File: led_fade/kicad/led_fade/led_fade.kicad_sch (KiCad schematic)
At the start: 3 parts

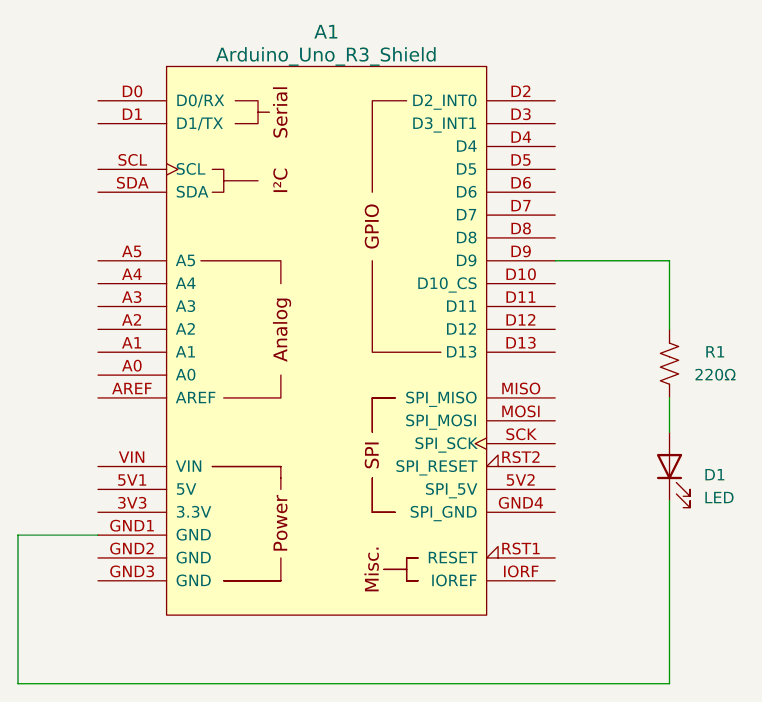
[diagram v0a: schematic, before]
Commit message: Use default Arduino UNO R3 symbol
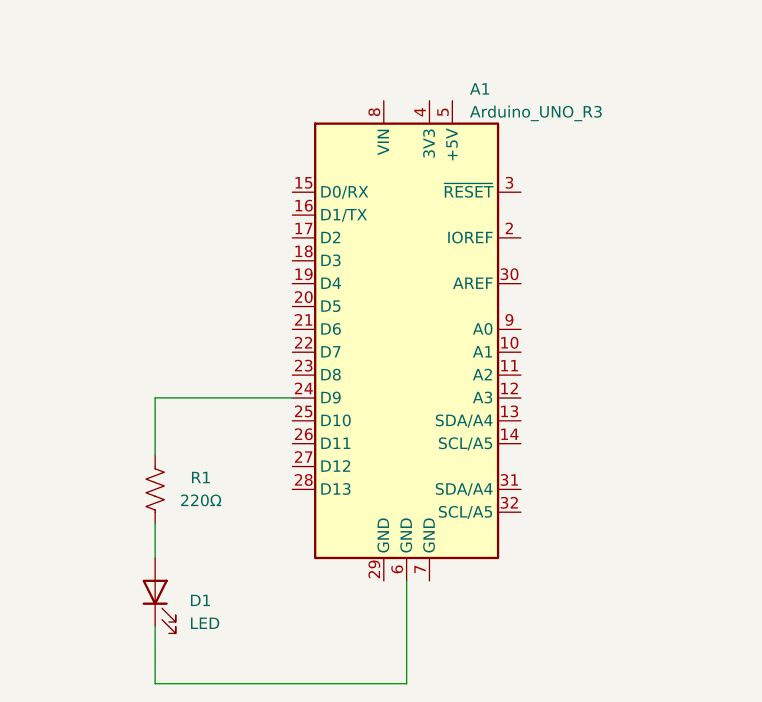
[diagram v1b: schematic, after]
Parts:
- removed A1: Arduino_Uno_R3_Shield, PCM_arduino-library:Arduino_Uno_R3_Shield, symbol PCM_arduino-library:Arduino_Uno_R3_Shield
- added A1: Arduino_UNO_R3, Module:Arduino_UNO_R3, symbol MCU_Module:Arduino_UNO_R3
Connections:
- net at R1.2: now also A1.24 (D9)
- net at D1.1 (K): now also A1.6 (GND)
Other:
- moved on the sheet: D1, R1
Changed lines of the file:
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@@
     (title "LED Fade")
   )
-  (wire (pts (xy 123.19 46.99) (xy 135.89 46.99))
+  (wire (pts (xy 78.74 93.98) (xy 78.74 87.63))
     (stroke (width 0) (type default))
   )
-  (wire (pts (xy 135.89 46.99) (xy 135.89 54.61))
+  (wire (pts (xy 106.68 82.55) (xy 106.68 93.98))
     (stroke (width 0) (type default))
   )
-  (wire (pts (xy 63.5 77.47) (xy 72.39 77.47))
+  (wire (pts (xy 78.74 62.23) (xy 78.74 68.58))
     (stroke (width 0) (type default))
   )
-  (wire (pts (xy 135.89 93.98) (xy 63.5 93.98))
+  (wire (pts (xy 106.68 93.98) (xy 78.74 93.98))
     (stroke (width 0) (type default))
   )
-  (wire (pts (xy 63.5 93.98) (xy 63.5 77.47))
+  (wire (pts (xy 93.98 62.23) (xy 78.74 62.23))
     (stroke (width 0) (type default))
   )
-  (wire (pts (xy 135.89 73.66) (xy 135.89 93.98))
+  (wire (pts (xy 78.74 76.2) (xy 78.74 80.01))
     (stroke (width 0) (type default))
   )
-  (wire (pts (xy 135.89 62.23) (xy 135.89 66.04))
-    (stroke (width 0) (type default))
-  )
-  (symbol (lib_id "PCM_arduino-library:Arduino_Uno_R3_Shield") (at 97.79 55.88 0) (unit 1)
-    (in_bom yes) (on_board yes) (dnp no) (fields_autoplaced)
-    (property "Reference" "A1" (at 97.79 21.59 0)
-      (effects (font (size 1.524 1.524)))
-    )
-    (property "Value" "Arduino_Uno_R3_Shield" (at 97.79 24.13 0)
-      (effects (font (size 1.524 1.524)))
-    )
-    (property "Footprint" "PCM_arduino-library:Arduino_Uno_R3_Shield" (at 97.79 93.98 0)
-      (effects (font (size 1.524 1.524)) hide)
-    )
-    (property "Datasheet" "https://docs.arduino.cc/hardware/uno-rev3" (at 97.79 90.17 0)
-      (effects (font (size 1.524 1.524)) hide)
-    )
-    (pin "3V3")
-    (pin "5V1")
-    (pin "5V2")
-    (pin "A0")
-    (pin "A1")
-    (pin "A2")
-    (pin "A3")
-    (pin "A4")
-    (pin "A5")
-    (pin "AREF")
-    (pin "D0")
-    (pin "D1")
-    (pin "D10")
-    (pin "D11")
-    (pin "D12")
-    (pin "D13")
-    (pin "D2")
-    (pin "D3")
-    (pin "D4")
-    (pin "D5")
-    (pin "D6")
-    (pin "D7")
-    (pin "D8")
-    (pin "D9")
-    (pin "GND1")
-    (pin "GND2")
-    (pin "GND3")
-    (pin "GND4")
-    (pin "IORF")
-    (pin "MISO")
-    (pin "MOSI")
-    (pin "RST1")
-    (pin "RST2")
-    (pin "SCK")
-    (pin "SCL")
-    (pin "SDA")
-    (pin "VIN")
-    (instances
-      (project "led_fade"
-        (path "/8b3a5294-7be8-49f2-a32e-5c19b07e6cc8"
-          (reference "A1") (unit 1)
-        )
-      )
-    )
-  )
-  (symbol (lib_id "Device:R_US") (at 135.89 58.42 180) (unit 1)
+  (symbol (lib_id "Device:R_US") (at 78.74 72.39 180) (unit 1)
     (in_bom yes) (on_board yes) (dnp no)
-    (property "Reference" "R1" (at 140.97 57.15 0)
+    (property "Reference" "R1" (at 83.82 71.12 0)
       (effects (font (size 1.27 1.27)))
     )
-    (property "Value" "220Ω" (at 140.97 59.69 0)
+    (property "Value" "220Ω" (at 83.82 73.66 0)
       (effects (font (size 1.27 1.27)))
     )
-    (property "Footprint" "" (at 134.874 58.166 90)
+    (property "Footprint" "" (at 77.724 72.136 90)
       (effects (font (size 1.27 1.27)) hide)
     )
-    (property "Datasheet" "~" (at 135.89 58.42 0)
+    (property "Datasheet" "~" (at 78.74 72.39 0)
       (effects (font (size 1.27 1.27)) hide)
     )
@@
     )
   )
-  (symbol (lib_id "Device:LED") (at 135.89 69.85 90) (unit 1)
+  (symbol (lib_id "Device:LED") (at 78.74 83.82 90) (unit 1)
     (in_bom yes) (on_board yes) (dnp no) (fields_autoplaced)
-    (property "Reference" "D1" (at 139.7 70.8025 90)
+    (property "Reference" "D1" (at 82.55 84.7725 90)
       (effects (font (size 1.27 1.27)) (justify right))
     )
-    (property "Value" "LED" (at 139.7 73.3425 90)
+    (property "Value" "LED" (at 82.55 87.3125 90)
       (effects (font (size 1.27 1.27)) (justify right))
     )
-    (property "Footprint" "" (at 135.89 69.85 0)
+    (property "Footprint" "" (at 78.74 83.82 0)
       (effects (font (size 1.27 1.27)) hide)
     )
-    (property "Datasheet" "~" (at 135.89 69.85 0)
+    (property "Datasheet" "~" (at 78.74 83.82 0)
       (effects (font (size 1.27 1.27)) hide)
     )
@@
         )
       )
+    )
+  )
+  (symbol (lib_id "MCU_Module:Arduino_UNO_R3") (at 106.68 54.61 0) (unit 1)
+    (in_bom yes) (on_board yes) (dnp no) (fields_autoplaced)
+    (property "Reference" "A1" (at 113.7159 27.94 0)
+      (effects (font (size 1.27 1.27)) (justify left))
+    )
+    (property "Value" "Arduino_UNO_R3" (at 113.7159 30.48 0)
+      (effects (font (size 1.27 1.27)) (justify left))
+    )
+    (property "Footprint" "Module:Arduino_UNO_R3" (at 106.68 54.61 0)
+      (effects (font (size 1.27 1.27) italic) hide)
+    )
+    (property "Datasheet" "https://www.arduino.cc/en/Main/arduinoBoardUno" (at 106.68 54.61 0)
+      (effects (font (size 1.27 1.27)) hide)
+    )
+    (pin "1")
+    (pin "10")
+    (pin "11")
+    (pin "12")
+    (pin "13")
+    (pin "14")
+    (pin "15")
+    (pin "16")
+    (pin "17")
+    (pin "18")
+    (pin "19")
+    (pin "2")
+    (pin "20")
+    (pin "21")
+    (pin "22")
+    (pin "23")
+    (pin "24")
+    (pin "25")
+    (pin "26")
+    (pin "27")
+    (pin "28")
+    (pin "29")
+    (pin "3")
+    (pin "30")
+    (pin "31")
+    (pin "32")
+    (pin "4")
+    (pin "5")
+    (pin "6")
+    (pin "7")
+    (pin "8")
+    (pin "9")
+    (instances
+      (project "led_fade"
+        (path "/8b3a5294-7be8-49f2-a32e-5c19b07e6cc8"
+          (reference "A1") (unit 1)
+        )
+      )
